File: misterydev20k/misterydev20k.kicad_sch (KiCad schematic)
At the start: 48 parts, among them J1 SWD, J2 USB_C_Receptacle_USB2.0, SW1 SW_Push, U10 TLV62569DBV, U2 W25Q128JVS, U3 USBLC6-2SC6, U4 RP2040, Y1 12MHz

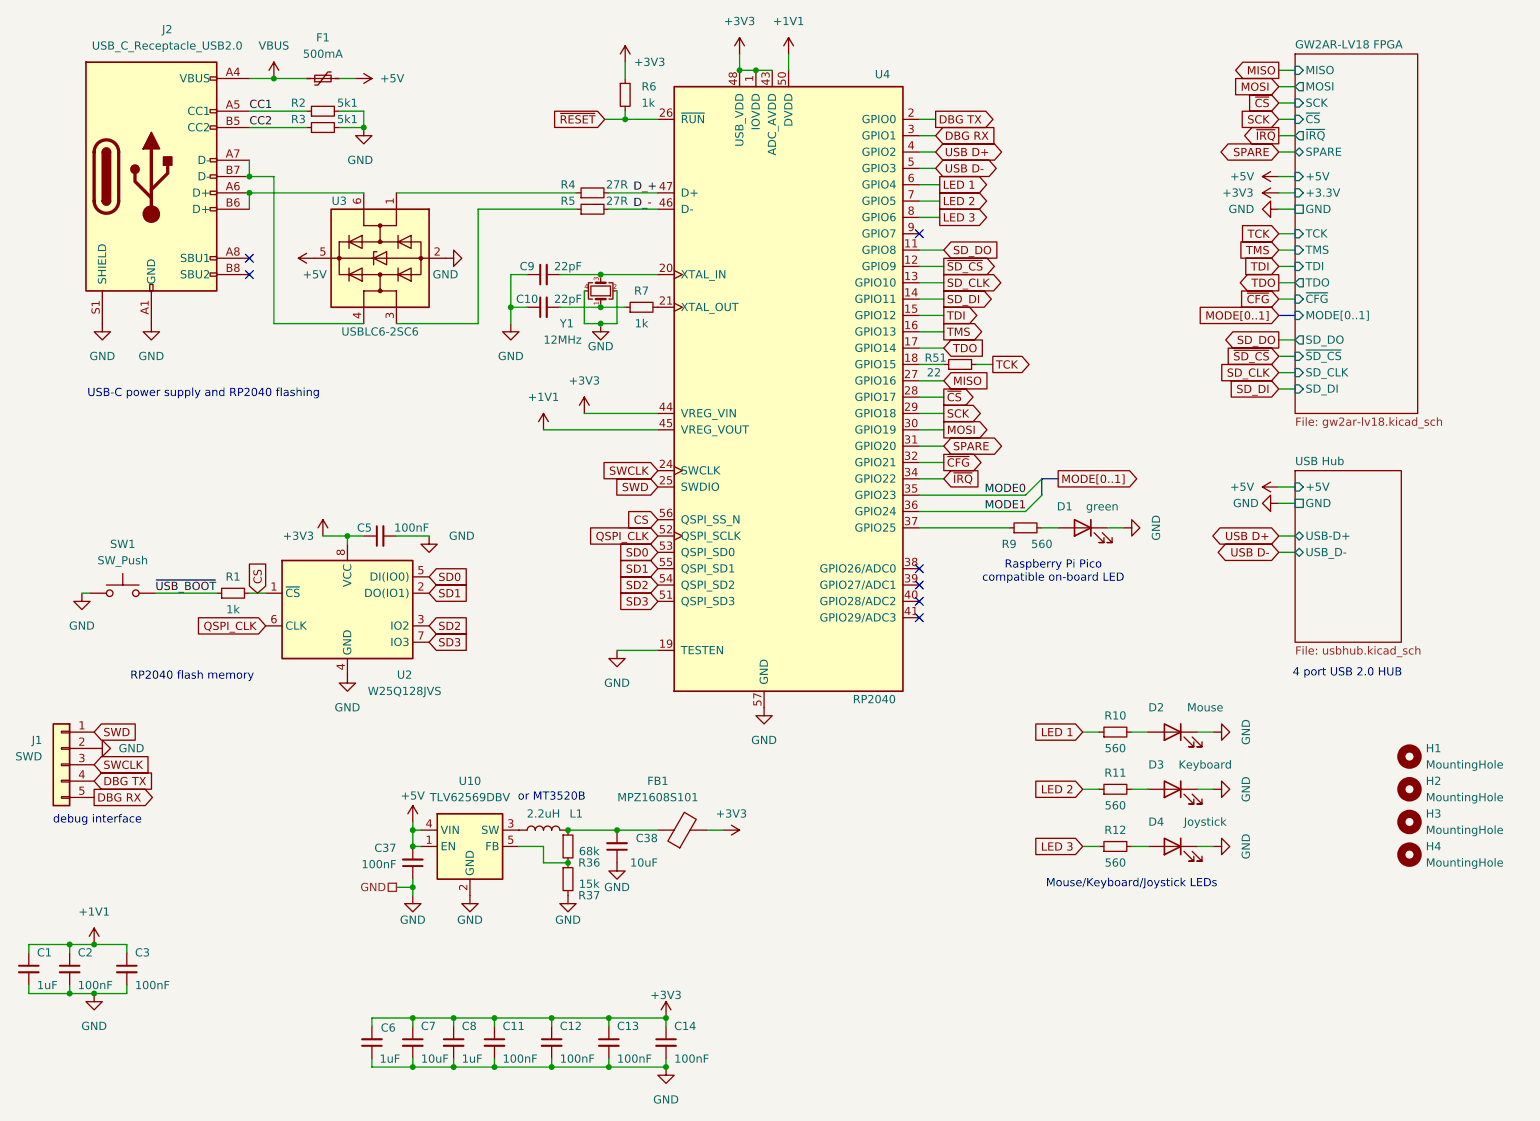
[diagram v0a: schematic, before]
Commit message: dev20k update
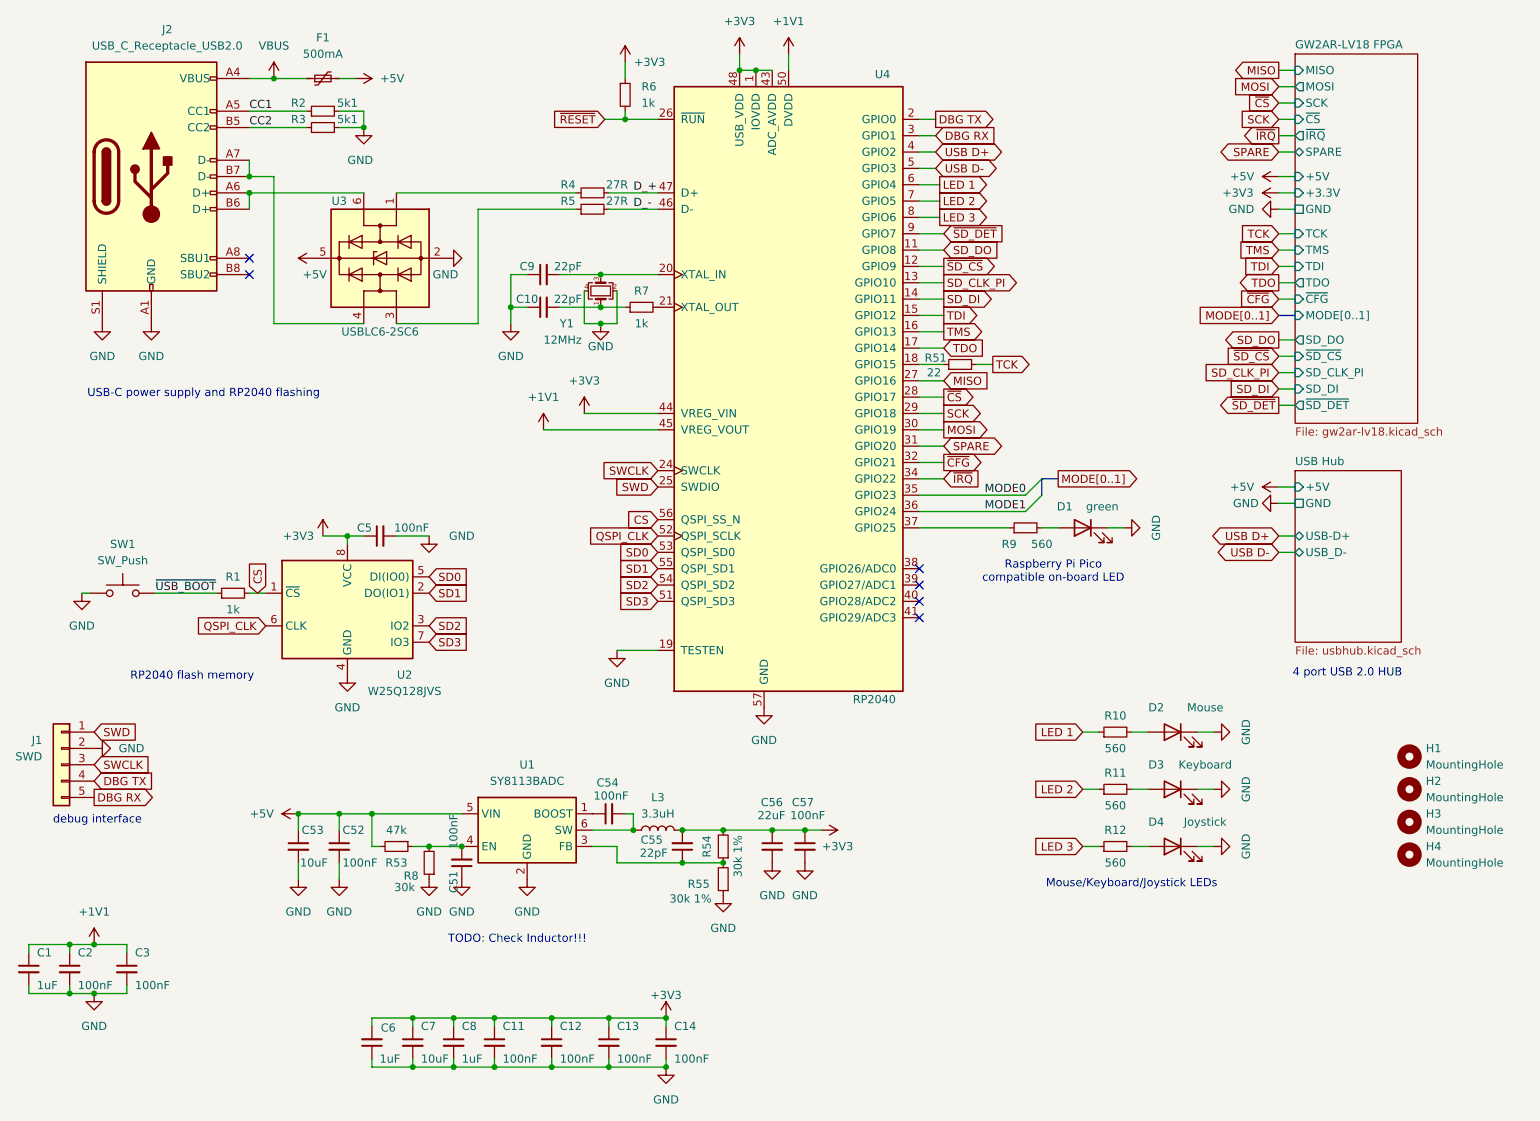
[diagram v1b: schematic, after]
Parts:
- removed C37: 100nF, Capacitor_SMD:C_0402_1005Metric, symbol Device:C_Small
- removed C38: 10uF, Capacitor_SMD:C_0402_1005Metric, symbol Device:C_Small
- removed FB1: MPZ1608S101, Inductor_SMD:L_0603_1608Metric, symbol Device:FerriteBead
- removed L1: 2.2uH, Inductor_SMD:L_0805_2012Metric, symbol Device:L
- removed R36: 68k, Resistor_SMD:R_0402_1005Metric, symbol Device:R_Small
- removed R37: 15k, Resistor_SMD:R_0402_1005Metric, symbol Device:R_Small
- removed U10: TLV62569DBV, Package_TO_SOT_SMD:SOT-23-5, symbol Regulator_Switching:TLV62569DBV
- added C51, C54: 100nF, Capacitor_SMD:C_0402_1005Metric, symbol Device:C_Small
- added C52, C57: 100nF, Capacitor_SMD:C_0603_1608Metric, symbol Device:C_Small
- added C53: 10uF, Capacitor_SMD:C_0603_1608Metric, symbol Device:C_Small
- added C55: 22pF, Capacitor_SMD:C_0402_1005Metric, symbol Device:C_Small
- added C56: 22uF, Capacitor_SMD:C_0603_1608Metric, symbol Device:C_Small
- added L3: 3.3uH, Inductor_SMD:L_Sunlord_MWSA0402S, symbol Device:L
- added R53: 47k, Resistor_SMD:R_0402_1005Metric, symbol Device:R_Small
- added R54, R55: 30k 1%, Resistor_SMD:R_0402_1005Metric, symbol Device:R_Small
- added R8: 30k, Resistor_SMD:R_0402_1005Metric, symbol Device:R_Small
- added U1: SY8113BADC, Package_TO_SOT_SMD:TSOT-23-6, symbol Regulator_Switching:LM2842Y
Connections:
- net +3V3: now also C55.2, C56.1, C57.1, L3.2, R54.2
- net +5V: now also C52.1, C53.1, R53.2, U1.5 (VIN)
- net GND: now also C51.1, C52.2, C53.2, C56.2, C57.2, R55.1, R8.1, U1.2 (GND)
- net ~{SD_DET}: now reaches U4.9 (GPIO7)
- net SD_CLK renamed SD_CLK_PI
- new net: C55.1, R54.1, R55.2, U1.3 (FB)
- new net: C54.1, U1.1 (BOOST)
- new net: C54.2, L3.1, U1.6 (SW)
- new net: C51.2, R53.1, R8.2, U1.4 (EN)
- no-connect marks 7 -> 6
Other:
- sheet GW2AR-LV18 FPGA ports: added SD_CLK_PI, ~{SD_DET}; removed SD_CLK
- note added: "TODO: Check Inductor!!!"
- note removed: "or MT3520B"
